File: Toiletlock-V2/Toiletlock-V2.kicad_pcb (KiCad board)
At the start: 2 copper layers, 100 x 100 mm, 33 parts, among them J1 Conn_ST_STDC14, J2 Conn_01x02_Male, J3 Conn_ARM_JTAG_SWD_20, SW1 SW_Push, U1 STM32G031K8T3, U2 DRV8837C, U3 APDS-9960, Y1 Crystal_GND24

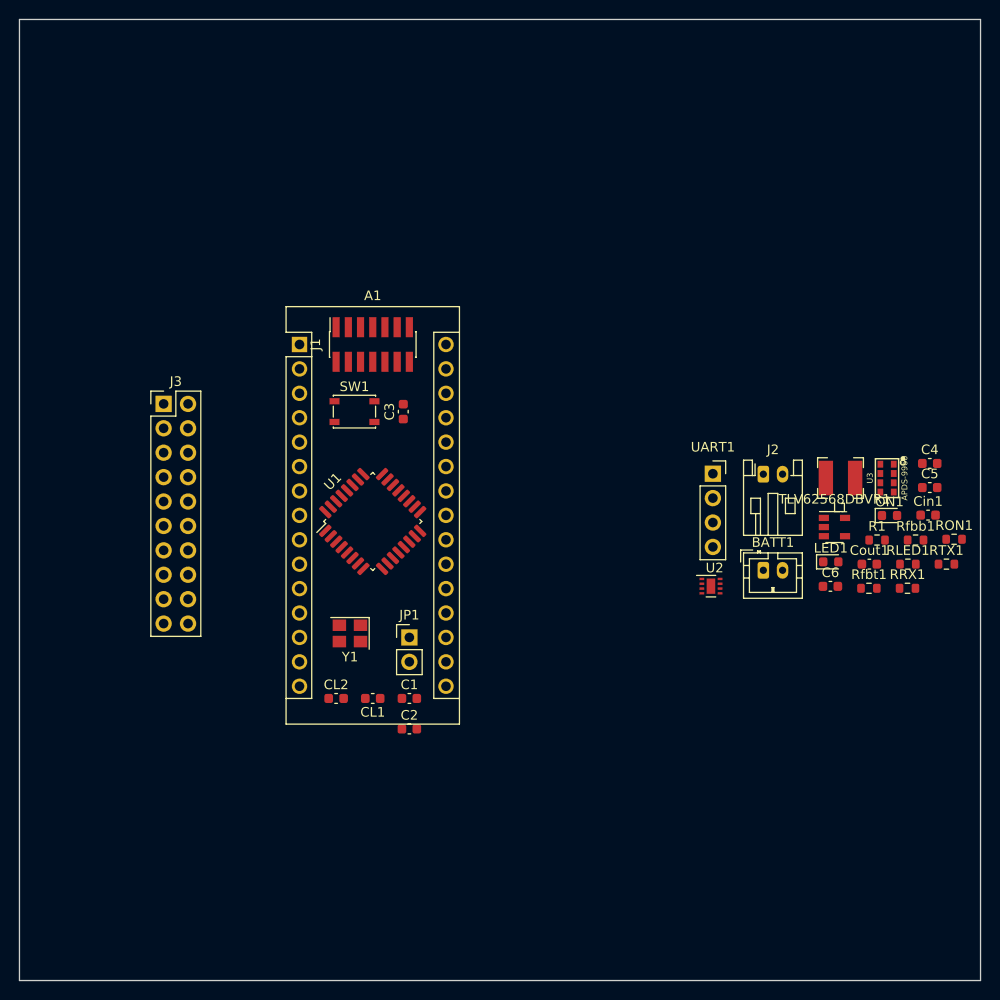
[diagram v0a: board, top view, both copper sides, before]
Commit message: Dev board finish
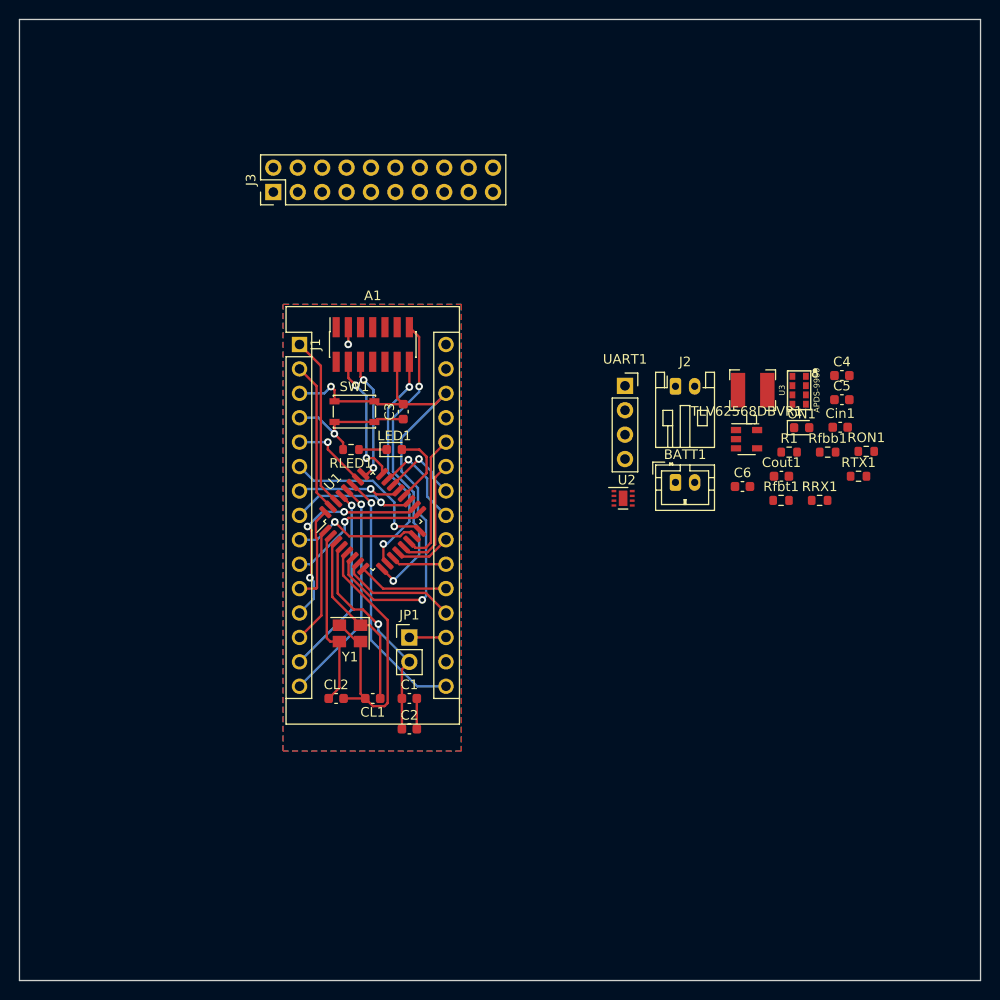
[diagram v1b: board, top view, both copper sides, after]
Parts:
- moved RLED1 59.2 mm to (134.5, 94.8), turned to 180 degrees
- moved LED1 46.9 mm to (139.0, 94.8)
- moved J3 24.8 mm to (126.4, 68.0), turned to 90 degrees
- moved C6 13.8 mm to (175.2, 98.6)
- moved Cin1 12.9 mm to (185.4, 92.4)
- moved L1 12.9 mm to (176.3, 88.6)
- moved RRX1 12.9 mm to (183.3, 100.0)
- moved Rfbb1 12.9 mm to (184.1, 95.0)
- moved U3 12.9 mm to (181.1, 88.6)
- moved UART1 12.9 mm to (163.0, 88.1)
- moved BATT1 12.9 mm to (168.3, 98.2)
- moved C4 12.9 mm to (185.6, 87.1)
- moved C5 12.9 mm to (185.6, 89.6)
- moved Cout1 12.9 mm to (179.3, 97.5)
- moved J2 12.9 mm to (168.3, 88.2)
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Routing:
- net /NRST: track 0.00 -> 57.4 mm, vias 0 -> 2
- net GND: track 0.00 -> 49.8 mm, vias 0 -> 1
- net T_VCP_TX: track 0.00 -> 31.9 mm, vias 0 -> 2
- net /PB3: track 0.00 -> 26.8 mm, vias 0 -> 1
- net VDD: track 0.00 -> 24.9 mm, vias 0 -> 2
- net T_VCP_RX: track 0.00 -> 24.3 mm, vias 0 -> 2
- net /PB4: track 0.00 -> 23.7 mm, vias 0 -> 1
- net /PA8: track 0.00 -> 22.1 mm, vias 0 -> 3
- net /PB5: track 0.00 -> 20.0 mm, vias 0 -> 1
- net Net-(CL1-Pad1): track 0.00 -> 19.1 mm
- net Net-(CL2-Pad1): track 0.00 -> 18.6 mm
- net /PB6: track 0.00 -> 17.9 mm
- net /PB1: track 0.00 -> 16.8 mm, vias 0 -> 1
- net /PB7: track 0.00 -> 15.7 mm
- net /PB2: track 0.00 -> 15.3 mm, vias 0 -> 1
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- added copper zone on F.Cu, net GND
- added copper zone on B.Cu, net VDD
